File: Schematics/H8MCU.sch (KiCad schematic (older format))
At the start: 8 parts

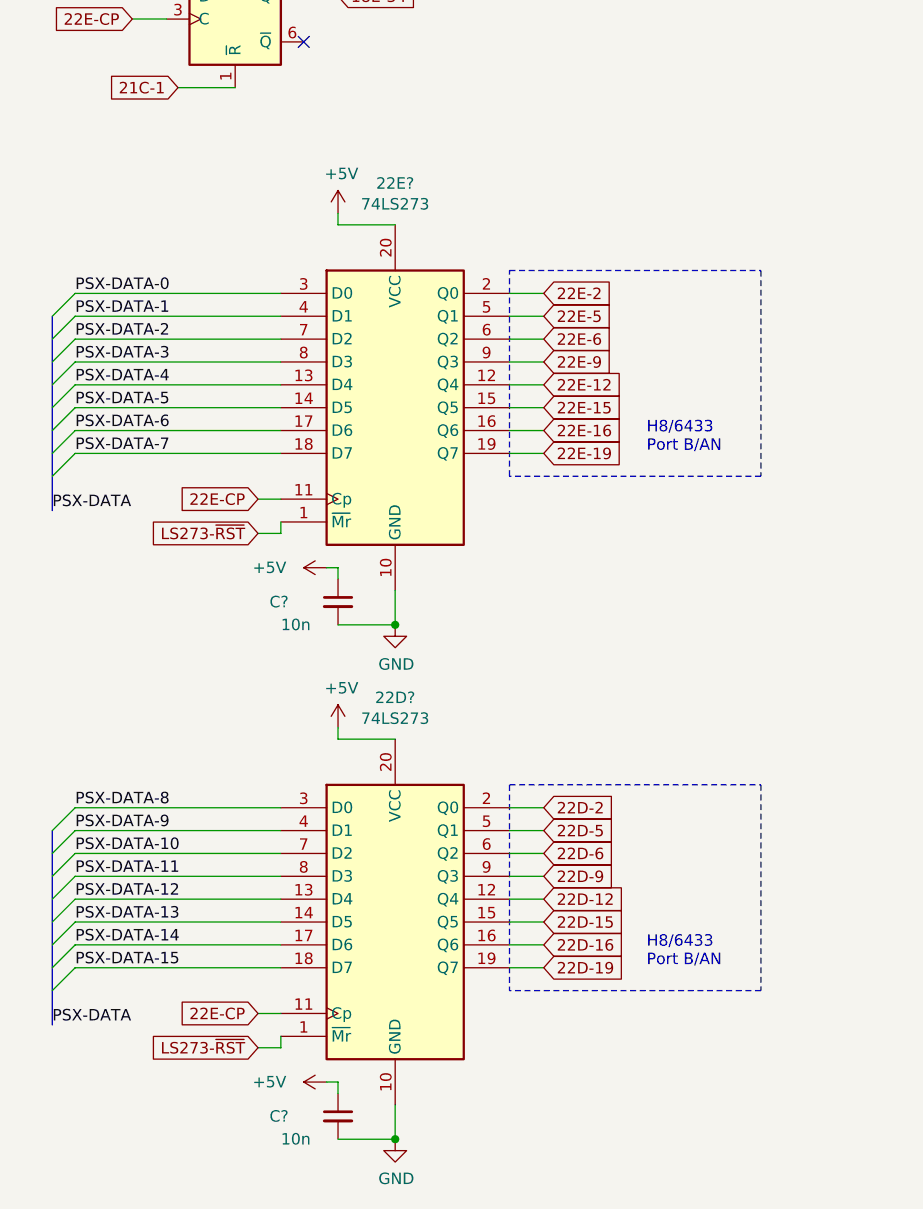
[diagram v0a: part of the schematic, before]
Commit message: Fixed bugs
IDE Retrace, PCMCIA checked
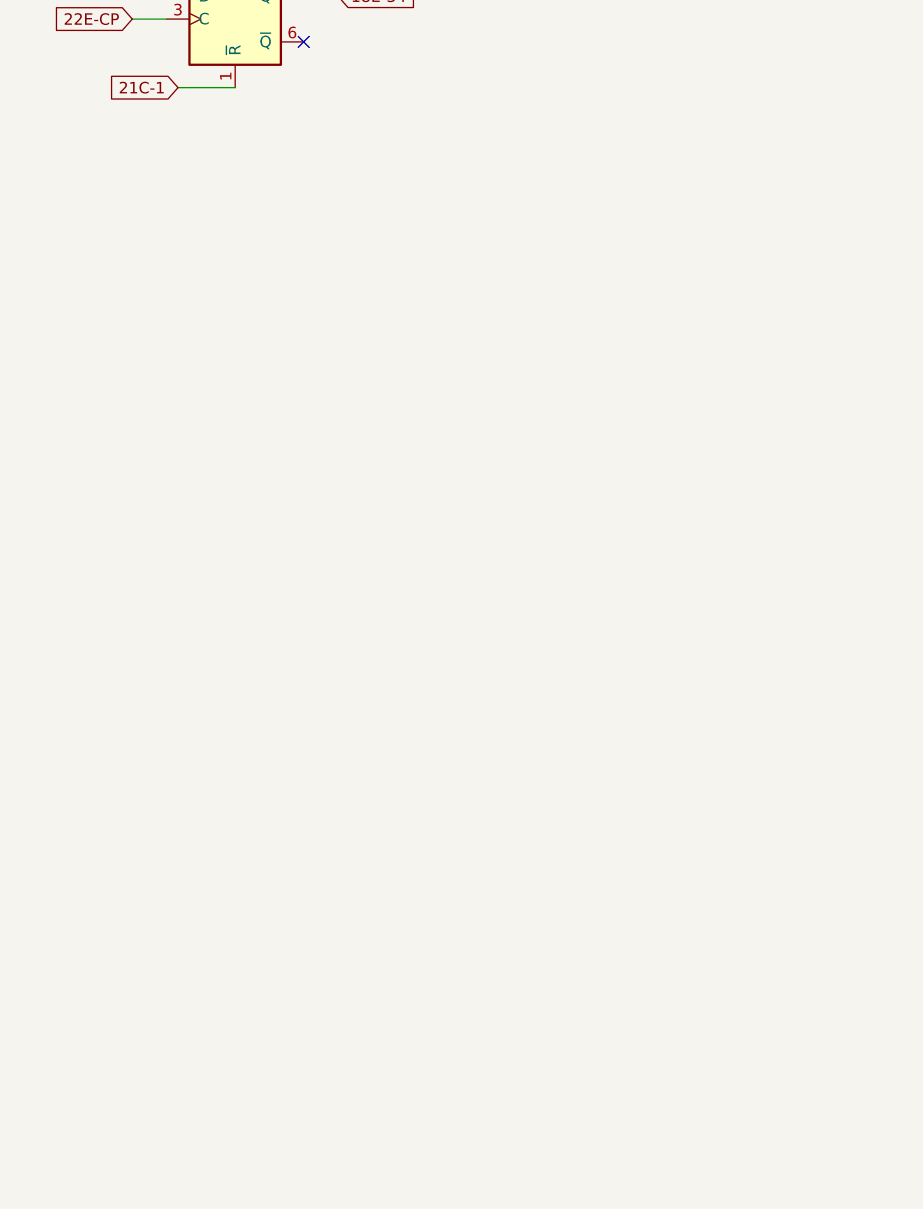
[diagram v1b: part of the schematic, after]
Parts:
- removed 22D?, 22E?: 74LS273, Package_SO:SO-20_5.3x12.6mm_P1.27mm, symbol 74xx:74LS273
- removed C? (x2): 10n, symbol Device:C_Small
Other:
- note removed: "H8/6433\nPort B/AN"
